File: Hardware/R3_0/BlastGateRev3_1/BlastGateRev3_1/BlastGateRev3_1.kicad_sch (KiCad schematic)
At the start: 42 parts, among them J1 Conn_01x03_Male, J2 Conn_01x06_Male, J3 USB_B_Micro, J4 RJ9, J5 Conn_01x03_Male, SW1 SW_DIP_x03, SW2 SW_SPDT_MSM, SW4 SW_SPDT_MSM, U1 AP2112M-3.3, U2 ESP32-WROOM-32D

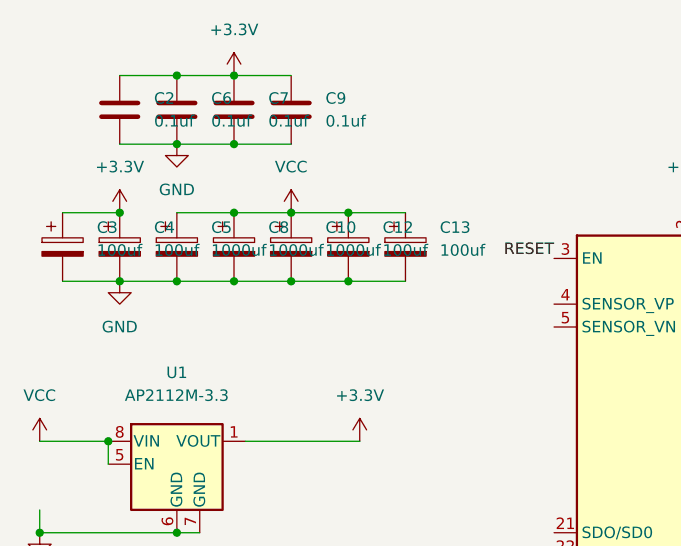
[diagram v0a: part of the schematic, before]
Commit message: hardware revision,
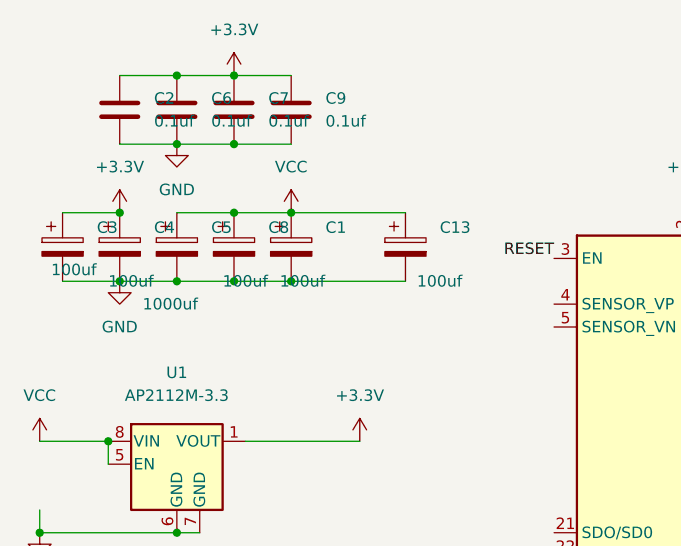
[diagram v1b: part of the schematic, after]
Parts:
- removed C10: 1000uf, Capacitor_THT:CP_Radial_D12.5mm_P5.00mm, symbol Device:C_Polarized
- removed C12: 100uf, Capacitor_THT:CP_Radial_D5.0mm_P2.50mm, symbol Device:C_Polarized
- added C1: 100uf, Capacitor_THT:CP_Radial_D5.0mm_P2.50mm, symbol Device:C_Polarized
- C8: value 1000uf -> 100uf; footprint Capacitor_THT:CP_Radial_D12.5mm_P5.00mm -> Capacitor_THT:CP_Radial_D5.0mm_P2.50mm
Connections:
- net GND: now also C1.2
- net VCC: now also C1.1
